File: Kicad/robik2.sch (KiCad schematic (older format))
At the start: 20 parts, among them J1 Conn_01x06_Male, J2 Conn_01x06_Male, J3 Conn_01x08_Male, J4 Conn_01x08_Male, J5 Conn_01x03_Male, Q1 BUZ11, SW1 Greenbtn, SW2 Resetbtn, SW3 Ebtn, SW4 Redbtn, U1 LM7805_TO220

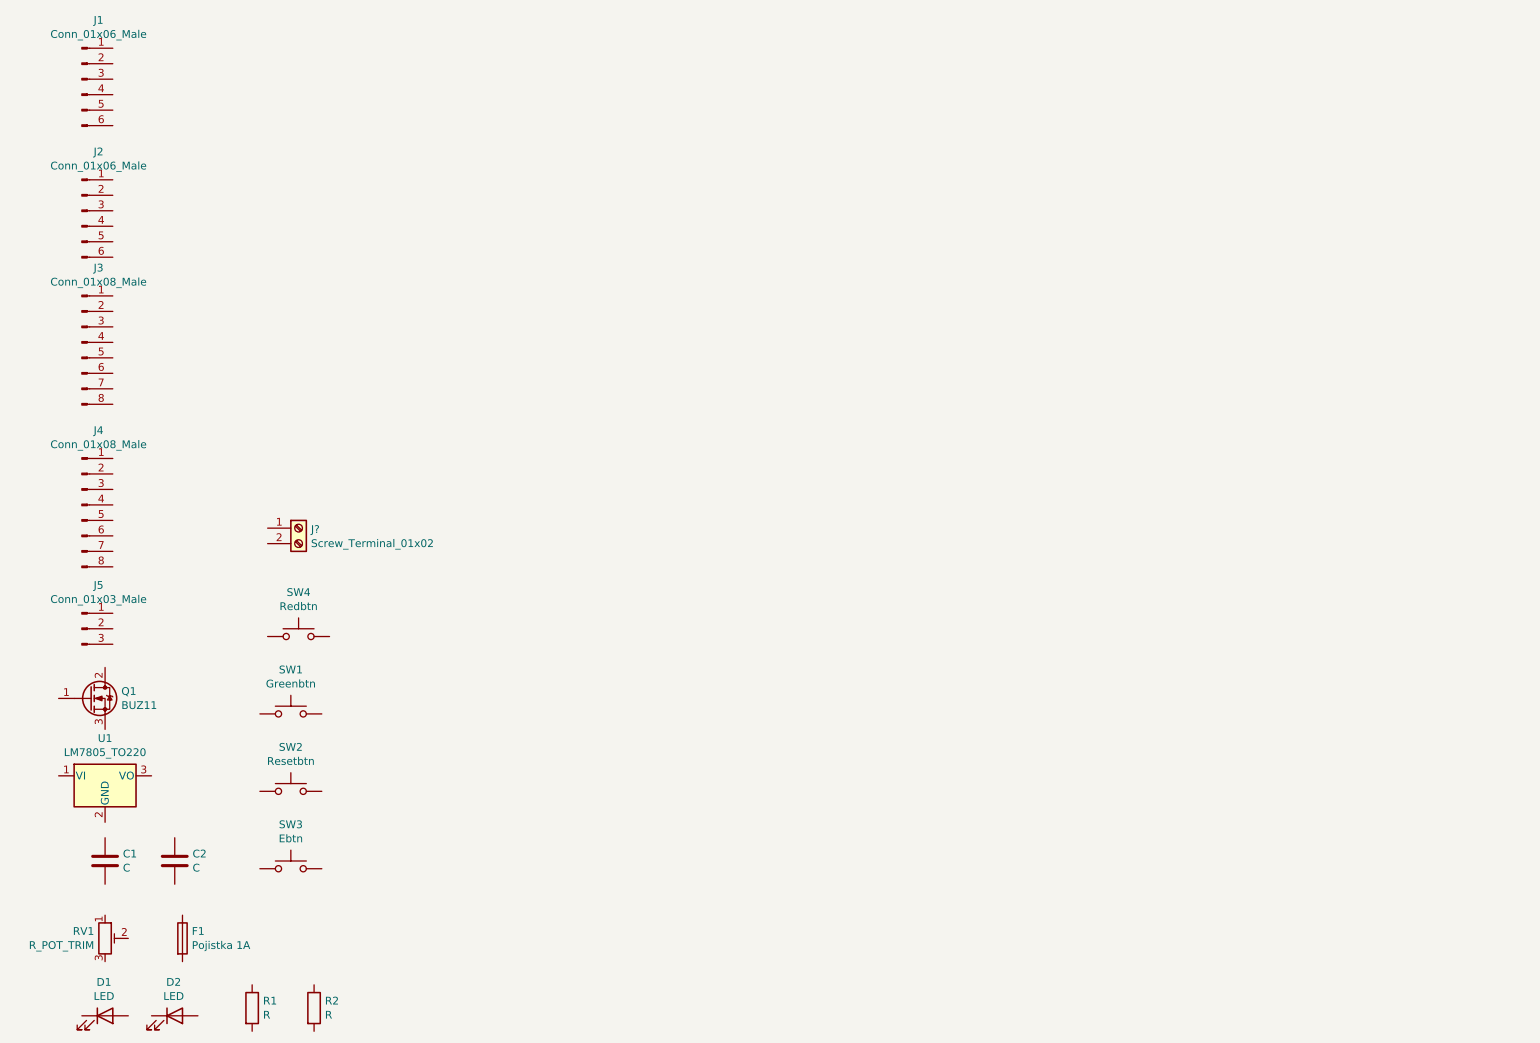
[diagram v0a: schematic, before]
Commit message: board
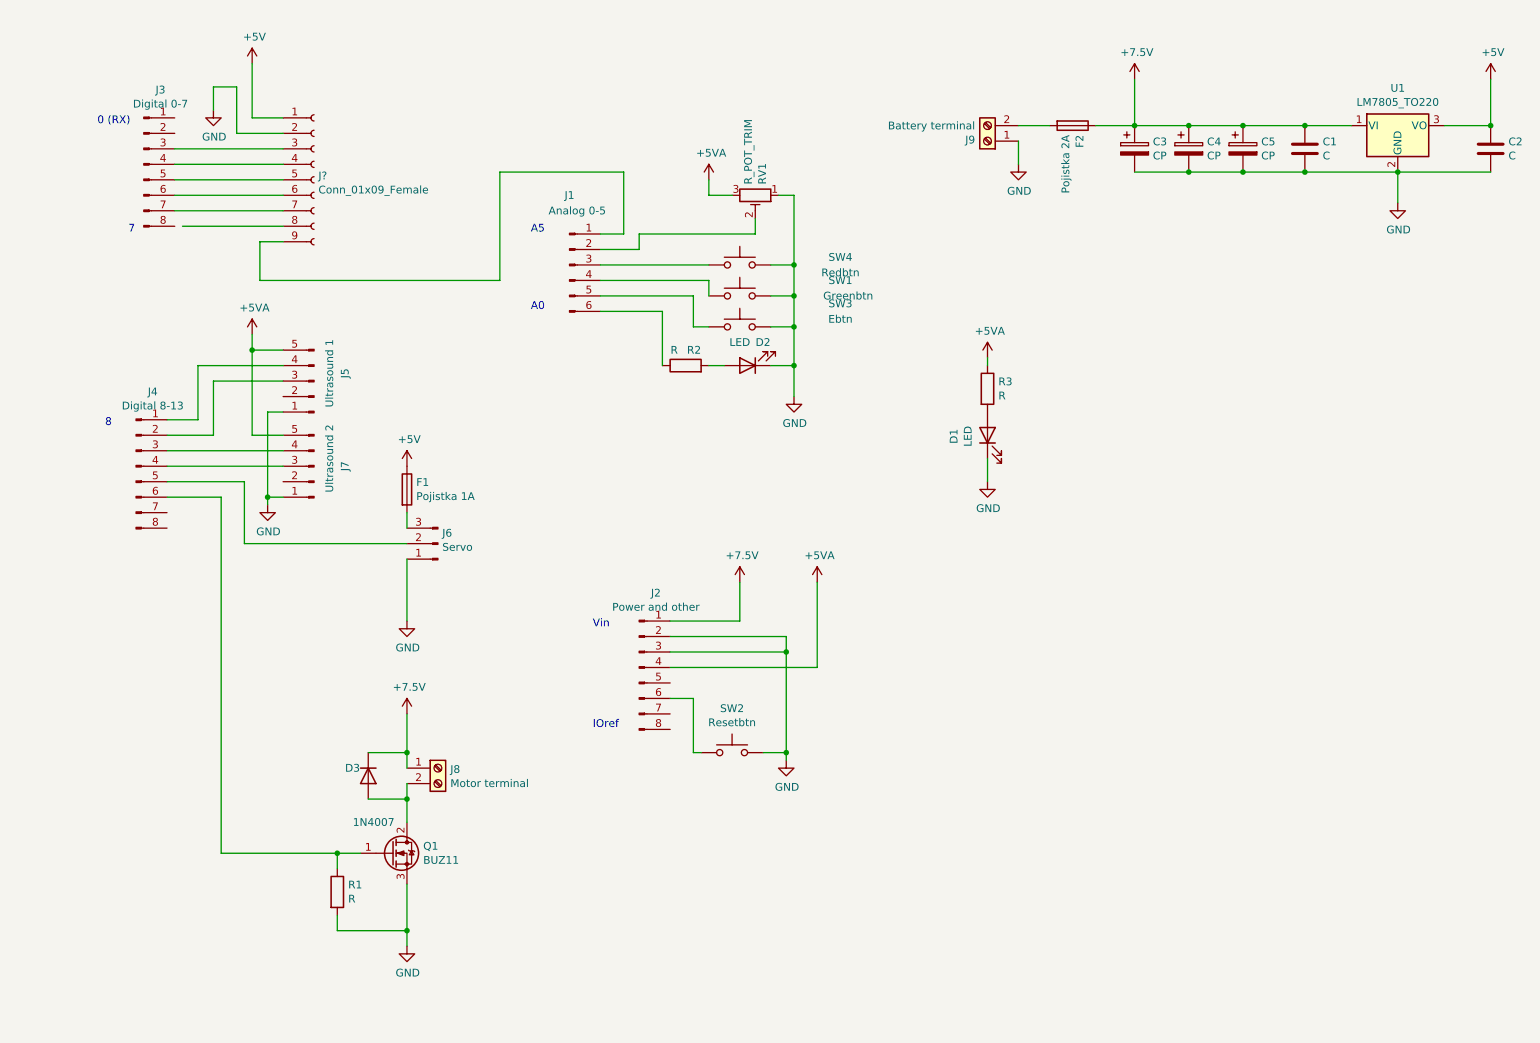
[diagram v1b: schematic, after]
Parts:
- removed J2: Conn_01x06_Male, Connector_PinSocket_2.00mm:PinSocket_1x06_P2.00mm_Vertical_SMD_Pin1Left, symbol Connector:Conn_01x06_Male
- removed J5: Conn_01x03_Male, Connector_PinSocket_2.00mm:PinSocket_1x03_P2.00mm_Vertical, symbol Connector:Conn_01x03_Male
- added C3, C4, C5: CP, Capacitor_THT:CP_Radial_D5.0mm_P2.00mm, symbol Device:CP
- added D3: 1N4007, Diode_THT:D_A-405_P10.16mm_Horizontal, symbol Device:D
- added F2: Pojistka 2A, Fuse:Fuse_sbeve, symbol Device:Fuse
- added J2: Power and other, Connector_PinSocket_2.00mm:PinSocket_1x08_P2.00mm_Vertical_SMD_Pin1Left, symbol Connector:Conn_01x08_Male
- added J5: Ultrasound 1, Connector_PinHeader_2.00mm:PinHeader_1x05_P2.00mm_Vertical, symbol Connector:Conn_01x05_Male
- added J6: Servo, Connector_PinHeader_2.00mm:PinHeader_1x03_P2.00mm_Vertical, symbol Connector:Conn_01x03_Male
- added J7: Ultrasound 2, Connector_PinHeader_2.00mm:PinHeader_1x05_P2.00mm_Vertical, symbol Connector:Conn_01x05_Male
- added J8: Motor terminal, TerminalBlock:TerminalBlock_bornier-2_P5.08mm, symbol Connector:Screw_Terminal_01x02
- added J?: Conn_01x09_Female, symbol Connector:Conn_01x09_Female
- added R3: R, Resistor_THT:R_Axial_DIN0207_L6.3mm_D2.5mm_P10.16mm_Horizontal, symbol Device:R
- F1: footprint Fuse:Fuseholder_Cylinder-5x20mm_Schurter_0031_8201_Horizontal_Open -> Fuse:Fuse_sbeve
- J1: value Conn_01x06_Male -> Analog 0-5
- J3: value Conn_01x08_Male -> Digital 0-7
- J4: value Conn_01x08_Male -> Digital 8-13
- J9: renamed from J?; value Screw_Terminal_01x02 -> Battery terminal; footprint (none) -> TerminalBlock:TerminalBlock_bornier-2_P5.08mm
- R1: footprint (none) -> Resistor_THT:R_Axial_DIN0207_L6.3mm_D2.5mm_P10.16mm_Horizontal
- R2: footprint (none) -> Resistor_THT:R_Axial_DIN0207_L6.3mm_D2.5mm_P7.62mm_Horizontal
- RV1: footprint Potentiometer_THT:Potentiometer_ACP_CA9-V10_Vertical_Hole -> Potentiometer_THT:Potentiometer_Runtron_RM-065_Vertical
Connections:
- net at J1.1 (Pin_1): now also J?.9 (Pin_9)
- net at J1.2 (Pin_2): now also RV1.2
- net at J1.3 (Pin_3): now also SW4.1
- net at J1.4 (Pin_4): now also SW1.1
- net at J1.5 (Pin_5): now also SW3.1
- net at J1.6 (Pin_6): now also R2.1
- net at J3.3 (Pin_3): now also J?.3 (Pin_3)
- net at J3.4 (Pin_4): now also J?.4 (Pin_4)
- net at J3.5 (Pin_5): now also J?.5 (Pin_5)
- net at J3.6 (Pin_6): now also J?.6 (Pin_6)
- net at J3.7 (Pin_7): now also J?.7 (Pin_7)
- net at J4.1 (Pin_1): now also J5.4 (Pin_4)
- net at J4.2 (Pin_2): now also J5.3 (Pin_3)
- net at J4.3 (Pin_3): now also J7.4 (Pin_4)
- net at J4.4 (Pin_4): now also J7.3 (Pin_3)
- net at J4.5 (Pin_5): now also J6.2 (Pin_2)
- net at J4.6 (Pin_6): now also Q1.1 (G), R1.1
- net at Q1.2 (D): now also D3.2 (A), J8.2 (Pin_2)
- net GND: now reaches Q1.3 (S)
- net GND: now also C1.2, C2.2, D1.1 (K), D2.1 (K), J9.1 (Pin_1), R1.2, RV1.1, SW1.2, SW2.2, SW3.2, SW4.2, U1.2 (GND), C3.2, C4.2, C5.2, J2.2 (Pin_2), J2.3 (Pin_3), J5.1 (Pin_1), J6.1 (Pin_1), J7.1 (Pin_1), J?.2 (Pin_2)
- net +7.5V: now reaches U1.1 (VI)
- net +7.5V: now also C1.1, C3.1, C4.1, C5.1, D3.1 (K), F2.1, J2.1 (Pin_1), J8.1 (Pin_1)
- net +5V: now reaches U1.3 (VO)
- net +5V: now also C2.1, F1.1, J?.1 (Pin_1)
- net +5VA: now reaches RV1.3
- net +5VA: now also J2.4 (Pin_4), J5.5 (Pin_5), J7.5 (Pin_5), R3.1
- net at D1.2 (A): now also R3.2
- net at D2.2 (A): now also R2.2
- net at F1.2: now also J6.3 (Pin_3)
- net at SW2.1: now also J2.6 (Pin_6)
- net at J9.2 (Pin_2): now also F2.2
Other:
- note added: "0 (RX)\n"
- note added: "7"
- note added: "8"
- note added: "A0"
- note added: "A5\n"
- note added: "IOref\n"
- note added: "Vin\n"
- moved on the sheet: C1, C2, D1, D2, F1, J1, J3, J4, J9, Q1, R1, R2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
